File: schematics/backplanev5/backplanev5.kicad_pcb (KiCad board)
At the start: 2 copper layers, 150 x 95 mm, 14 parts, among them J11 Conn_01x02, J12 Conn_01x02, J13 Conn_01x02, J14 Conn_01x02

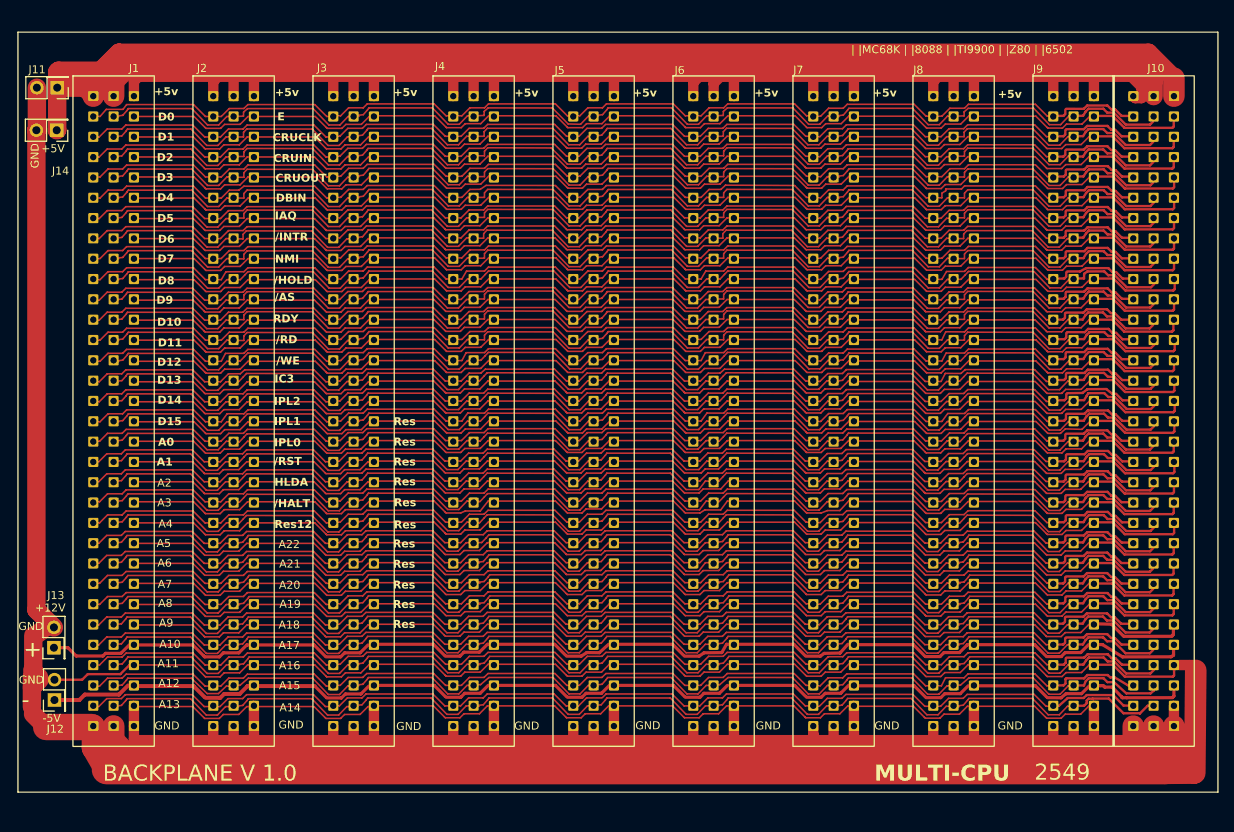
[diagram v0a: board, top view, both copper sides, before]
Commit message: Update V1 fabrication 04-12-2025 JLCPCB
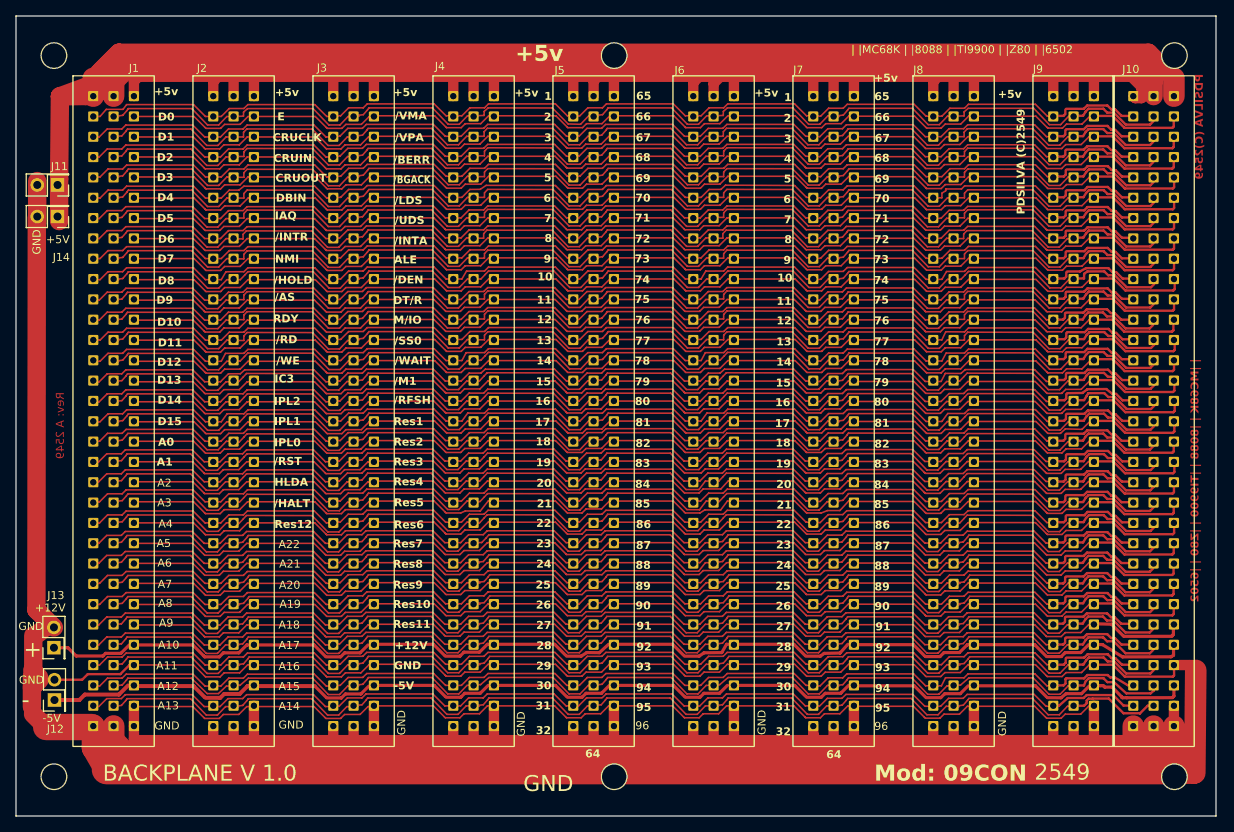
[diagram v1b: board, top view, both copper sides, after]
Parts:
- added H1: MountingHole, MountingHole:MountingHole_3.2mm_M3, F.Cu at (20.0, 24.9)
- added H2: MountingHole, MountingHole:MountingHole_3.2mm_M3, F.Cu at (20.0, 115.1)
- added H3: MountingHole, MountingHole:MountingHole_3.2mm_M3, F.Cu at (160.1, 115.1)
- added H4: MountingHole, MountingHole:MountingHole_3.2mm_M3, F.Cu at (160.1, 24.9)
- added H5: MountingHole, MountingHole:MountingHole_3.2mm_M3, F.Cu at (90.0, 24.9)
- added H6: MountingHole, MountingHole:MountingHole_3.2mm_M3, F.Cu at (90.0, 115.1)
- moved J11 12.2 mm to (20.5, 41.1)
- moved J14 10.8 mm to (20.5, 45.0)
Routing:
- net GND: track 874.4 -> 863.4 mm
- net /backplane/+5V: track 490.3 -> 499.6 mm
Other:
- board size 150 x 95 mm -> 150 x 100 mm
- board text added: "/BERR"
- board text added: "/BGACK"
- board text added: "/DEN"
- board text added: "/INTA"
- board text added: "/LDS"
- board text added: "/M1"
- board text added: "/RFSH"
- board text added: "/SS0"
- board text added: "/UDS"
- board text added: "/VMA"
- board text added: "/VPA"
- board text added: "/WAIT"
- board text added: "1"
- board text added: "10"
- board text added: "11"
- board text added: "12"
- board text added: "13"
- board text added: "14"
- board text added: "15"
- board text added: "16"
- board text added: "17"
- board text added: "18"
- board text added: "19"
- board text added: "2"
- board text added: "20"
- board text added: "21"
- board text added: "22"
- board text added: "23"
- board text added: "24"
- board text added: "25"
- board text added: "26"
- board text added: "27"
- board text added: "28"
- board text added: "29"
- board text added: "3"
- board text added: "30"
- board text added: "31"
- board text added: "32"
- board text added: "4"
- board text added: "5"
- board text added: "6"
- board text added: "64"
- board text added: "65"
- board text added: "66"
- board text added: "67"
- board text added: "68"
- board text added: "69"
- board text added: "7"
- board text added: "70"
- board text added: "71"
- board text added: "72"
- board text added: "73"
- board text added: "74"
- board text added: "75"
- board text added: "76"
- board text added: "77"
- board text added: "78"
- board text added: "79"
- board text added: "8"
- board text added: "80"
- board text added: "81"
- board text added: "82"
- board text added: "83"
- board text added: "84"
- board text added: "85"
- board text added: "86"
- board text added: "87"
- board text added: "88"
- board text added: "89"
- board text added: "9"
- board text added: "90"
- board text added: "91"
- board text added: "92"
- board text added: "93"
- board text added: "94"
- board text added: "95"
- board text added: "96"
- board text added: "ALE"
- board text added: "DT/R"
- board text added: "M/IO"
- board text added: "Mod: 09CON"
- board text added: "PDSILVA (C)2549"
- board text added: "Res1"
- board text added: "Res10"
- board text added: "Res11"
- board text added: "Res2"
- board text added: "Res3"
- board text added: "Res4"
- board text added: "Res5"
- board text added: "Res6"
- board text added: "Res7"
- board text added: "Res8"
- board text added: "Res9"
- board text added: "Rev: A 2549"
- board text removed: "MULTI-CPU"
- board text removed: "Res"
